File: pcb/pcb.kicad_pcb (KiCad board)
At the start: 2 copper layers, 88.8 x 45.1 mm, 14 parts, among them SW1 SW_Push, SW2 SW_Push, SW3 SW_Push, SW4 SW_Push, SW5 RotaryEncoder_Switch, U1 XIAO-RP2040-DIP

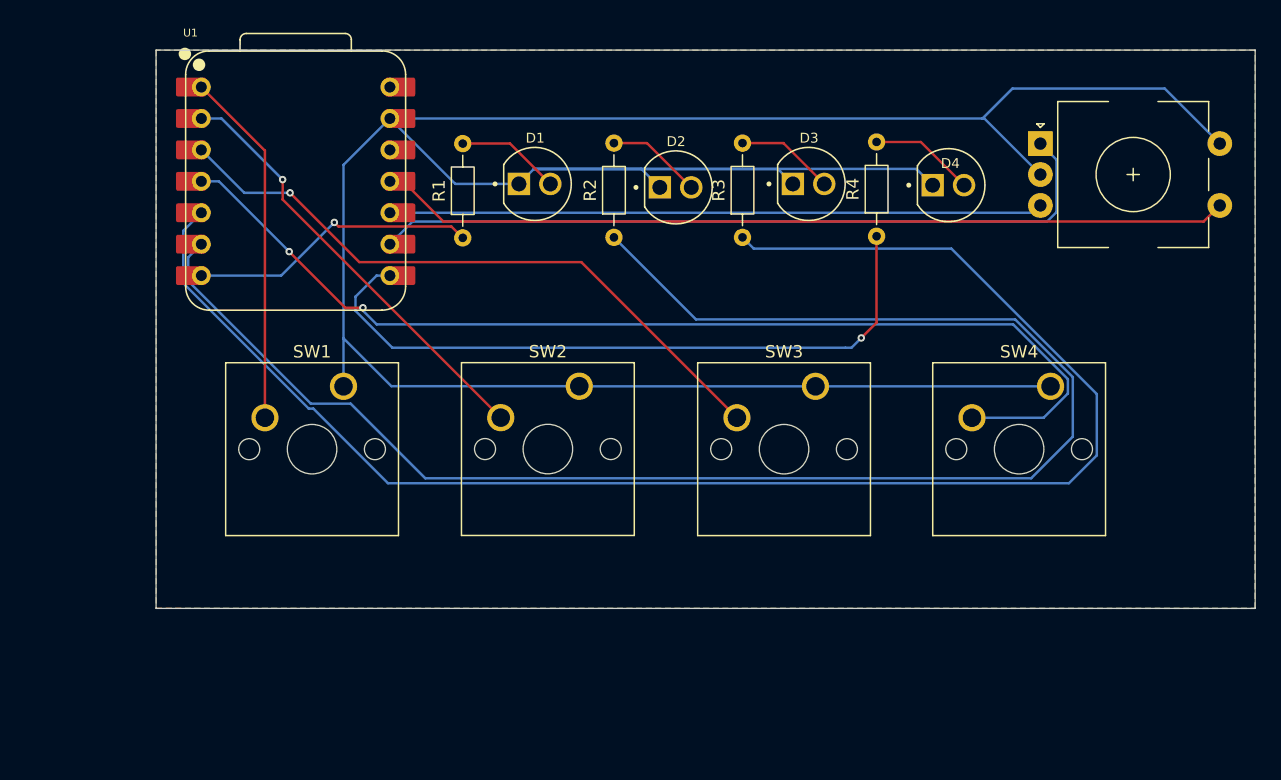
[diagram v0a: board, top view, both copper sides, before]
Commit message: updated pcb
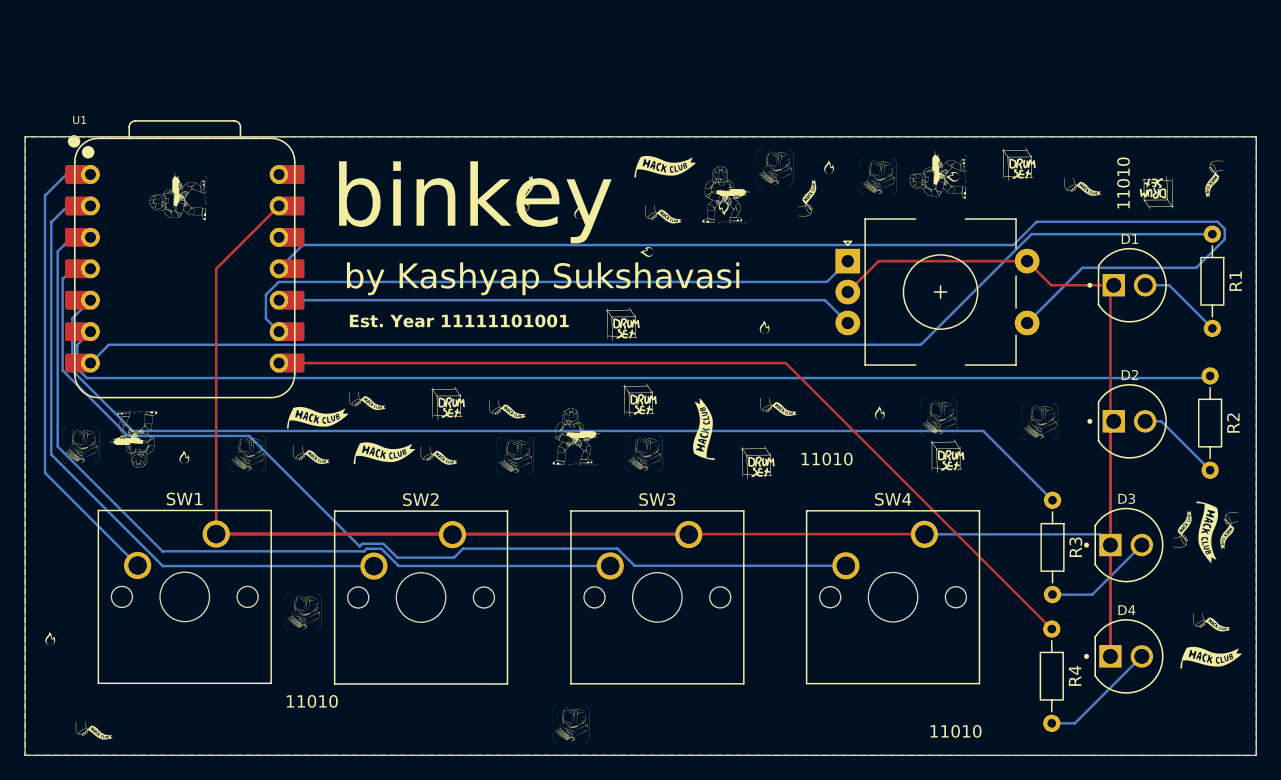
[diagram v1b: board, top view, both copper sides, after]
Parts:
- added G***: LOGO, xiaorp2040:computer, F.Cu at (57.5, 95.0)
- added G***: LOGO, xiaorp2040:fir, F.Cu at (118.0, 72.4)
- added G***: LOGO, xiaorp2040:drum, F.Cu at (127.5, 95.8)
- added G***: LOGO, xiaorp2040:orphSmall, F.Cu at (93.5, 74.6)
- added G***: LOGO, xiaorp2040:orphSmall, F.Cu at (92.0, 92.1)
- added G***: LOGO, xiaorp2040:orphSmall, F.Cu at (80.7, 91.5)
- added G***: LOGO, xiaorp2040:flagSmall, F.Cu at (82.1, 95.6)
- added G***: LOGO, xiaorp2040:fir, F.Cu at (128.0, 73.2)
- added G***: LOGO, xiaorp2040:computer, F.Cu at (135.0, 93.0)
- added G***: LOGO, xiaorp2040:misterChiefSmal, F.Cu at (61.8, 94.5)
- added G***: LOGO, xiaorp2040:computer, F.Cu at (103.0, 95.6)
- added G***: LOGO, xiaorp2040:drum, F.Cu at (144.5, 74.6)
- added G***: LOGO, xiaorp2040:flagSmall, F.Cu at (76.7, 92.7)
- added G***: LOGO, xiaorp2040:misterChiefSmal, F.Cu at (97.5, 94.2)
- added G***: LOGO, xiaorp2040:fir, F.Cu at (103.2, 79.3)
- added G***: LOGO, xiaorp2040:orphSmall, F.Cu at (116.3, 75.0)
- added G***: LOGO, xiaorp2040:fir, F.Cu at (97.8, 76.1)
- added G***: LOGO, xiaorp2040:drum, F.Cu at (133.3, 72.2)
- added G***: LOGO, xiaorp2040:orphSmall, F.Cu at (150.2, 101.8)
- added G***: LOGO, xiaorp2040:misterChiefSmal, F.Cu at (109.6, 74.7)
- added G***: LOGO, xiaorp2040:orphSmall, F.Cu at (113.9, 91.9)
- added G***: LOGO, xiaorp2040:computer, F.Cu at (97.1, 117.5)
- added G***: LOGO, xiaorp2040:computer, F.Cu at (75.5, 108.4)
- added G***: LOGO, xiaorp2040:misterChiefSmal, F.Cu at (65.3, 74.9)
- added G***: LOGO, xiaorp2040:orphSmall, F.Cu at (146.7, 101.7)
- added G***: LOGO, xiaorp2040:orphSmall, F.Cu at (86.5, 95.9)
- added G***: LOGO, xiaorp2040:flagSmall, F.Cu at (107.9, 93.6)
- added G***: LOGO, xiaorp2040:drum, F.Cu at (112.2, 96.3)
- added G***: LOGO, xiaorp2040:orphSmall, F.Cu at (58.6, 118.1)
- added G***: LOGO, xiaorp2040:orphSmall, F.Cu at (76.1, 95.8)
- added G***: LOGO, xiaorp2040:fir, F.Cu at (65.9, 95.9)
- added G***: LOGO, xiaorp2040:orphSmall, F.Cu at (149.0, 73.4)
- added G***: LOGO, xiaorp2040:orphSmall, F.Cu at (138.5, 74.1)
- added G***: LOGO, xiaorp2040:computer, F.Cu at (121.9, 73.2)
- added G***: LOGO, xiaorp2040:computer, F.Cu at (92.6, 95.8)
- added G***: LOGO, xiaorp2040:orphSmall, F.Cu at (148.9, 109.4)
- added G***: LOGO, xiaorp2040:fir, F.Cu at (112.8, 85.4)
- added G***: LOGO, xiaorp2040:fir, F.Cu at (122.1, 92.3)
- added G***: LOGO, xiaorp2040:fir, F.Cu at (55.0, 110.5)
- added G***: LOGO, xiaorp2040:computer, F.Cu at (113.6, 72.5)
- added G***: LOGO, xiaorp2040:drum, F.Cu at (101.3, 85.1)
- added G***: LOGO, xiaorp2040:misterChiefSmal, F.Cu at (126.8, 73.1)
- added G***: LOGO, xiaorp2040:flagSmall, F.Cu at (148.6, 102.0)
- added G***: LOGO, xiaorp2040:drum, F.Cu at (102.7, 91.2)
- added G***: LOGO, xiaorp2040:orphSmall, F.Cu at (104.6, 76.4)
- added G***: LOGO, xiaorp2040:flagSmall, F.Cu at (148.9, 112.1)
- added G***: LOGO, xiaorp2040:computer, F.Cu at (71.0, 95.6)
- added G***: LOGO, xiaorp2040:awpmid, B.Cu at (100.7, 88.0)
- added G***: LOGO, xiaorp2040:drum, F.Cu at (87.2, 91.5)
- added G***: LOGO, xiaorp2040:fir, F.Cu at (109.5, 75.8)
- added G***: LOGO, xiaorp2040:flagSmall, F.Cu at (104.8, 72.4)
- added G***: LOGO, xiaorp2040:computer, F.Cu at (126.8, 92.7)
- moved R1 60.6 mm to (149.0, 77.9), turned to -90 degrees
- moved R2 49.5 mm to (148.8, 89.3), turned to -90 degrees
- moved D1 48.8 mm to (142.3, 82.0)
- moved D2 41.3 mm to (142.3, 93.0)
- moved D4 40.7 mm to (142.0, 112.0)
- moved D3 38.9 mm to (142.0, 103.0)
- moved R4 34.8 mm to (136.0, 109.8), turned to -90 degrees
- moved R3 32.9 mm to (136.1, 99.4), turned to -90 degrees
- moved SW5 18.2 mm to (127.0, 82.5)
- moved SW2 15.8 mm to (87.5, 102.2)
- moved SW1 15.8 mm to (68.5, 102.1)
- moved SW3 15.8 mm to (106.7, 102.2)
- moved SW4 15.7 mm to (125.7, 102.1)
- moved U1 11.4 mm to (65.9, 80.7)
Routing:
- net Net-(U1-GPIO0/TX): track 24.3 -> 95.0 mm, vias 1 -> 0
- net Net-(U1-GPIO6/SDA): track 126.6 -> 89.9 mm
- net Net-(U1-GPIO7/SCL): track 129.5 -> 95.4 mm
- net Net-(U1-GPIO3/MOSI): track 69.0 -> 97.9 mm
- net Net-(U1-GPIO27/ADC1/A1): track 35.2 -> 52.3 mm, vias 1 -> 0
- net Net-(U1-GPIO1/RX): track 55.8 -> 71.4 mm, vias 1 -> 0
- net Net-(U1-GPIO28/ADC2/A2): track 52.3 -> 67.7 mm, vias 1 -> 0
- net Net-(U1-GPIO2/SCK): track 61.0 -> 51.6 mm
- net Net-(U1-GPIO26/ADC0/A0): track 28.9 -> 37.4 mm
- net Net-(U1-GPIO4/MISO): track 52.8 -> 46.7 mm
- net Net-(U1-GPIO29/ADC3/A3): track 86.6 -> 80.6 mm, vias 2 -> 0
- net GND: track 237.8 -> 240.2 mm
- net Net-(D1-PadA): track 8.43 -> 6.88 mm
- net Net-(D4-PadA): track 8.52 -> 9.52 mm
- net Net-(D3-PadA): track 7.98 -> 8.88 mm
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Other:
- board size 88.8 x 45.1 mm -> 99.5 x 50 mm
- board text added: "$15, 233.40"
- board text added: "11010"
- board text added: "AWP | Dragon Lore"
- board text added: "Est. Year 11111101001"
- board text added: "binkey"
- board text added: "by Kashyap Sukshavasi"
- board text added: "{dblquote}Becase bread taste better than key{dblquote} - Instagram Dude"
- board text added: "{dblquote}Were it so easy...{dblquote} - Thel 'Vadam, Halo 3"
- board text added: "{dblquote}You don't have to be the greatest Omni-Man ever. You just have to be the greatest you.{dblquote} - Debbie Grayson to Mark Grayson (Invincible)"
